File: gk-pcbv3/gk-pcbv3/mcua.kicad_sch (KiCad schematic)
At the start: 24 parts, among them J14 Conn_01x02, SW1 SW_Push, U4 STM32H747BITx, Y1 16MHz, Y2 32.768kHz R26-32.768-12.5

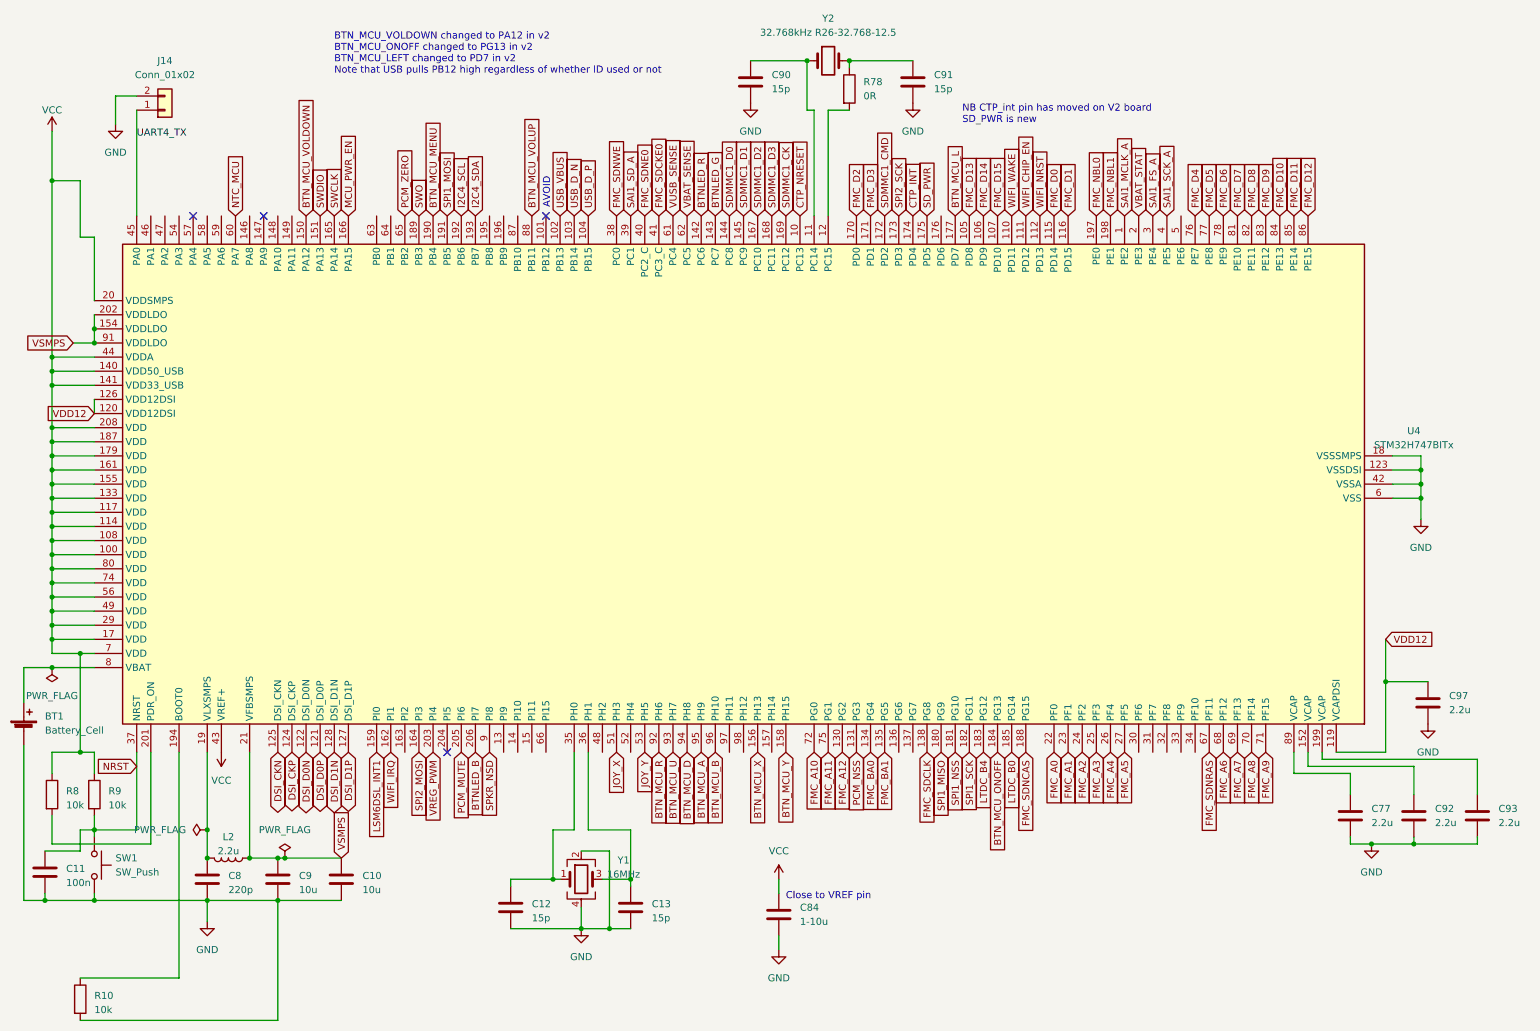
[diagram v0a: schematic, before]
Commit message: v3 board
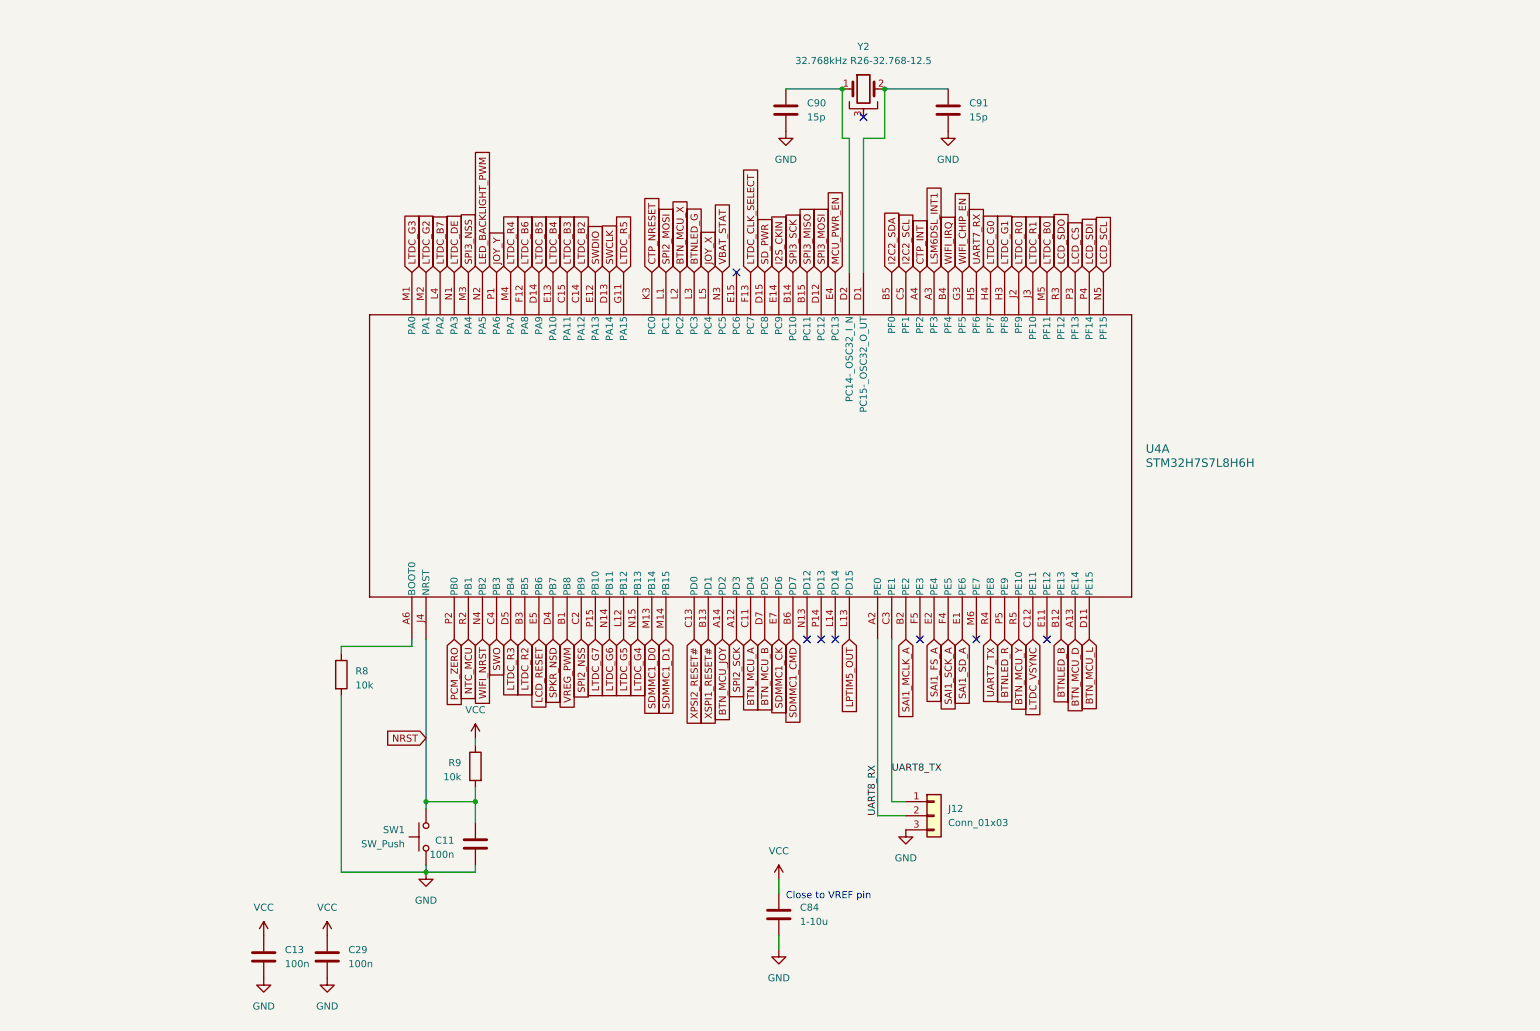
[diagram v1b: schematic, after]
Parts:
- removed BT1: Battery_Cell, Battery:BatteryHolder_Keystone_3002_1x2032, symbol Device:Battery_Cell
- removed C10, C9: 10u, Capacitor_SMD:C_0805_2012Metric, symbol Device:C
- removed C12: 15p, Capacitor_SMD:C_0603_1608Metric, symbol Device:C
- removed C77, C92, C93: 2.2u, Capacitor_SMD:C_0603_1608Metric, symbol Device:C
- removed C8: 220p, Capacitor_SMD:C_0603_1608Metric, symbol Device:C
- removed C97: 2.2u, Capacitor_SMD:C_0805_2012Metric, symbol Device:C
- removed J14: Conn_01x02, Connector_PinHeader_2.54mm:PinHeader_1x02_P2.54mm_Vertical, symbol Connector_Generic:Conn_01x02
- removed L2: 2.2u, Inductor_SMD:L_7.3x7.3_H3.5, symbol Device:L
- removed R10: 10k, Resistor_SMD:R_0603_1608Metric, symbol Device:R
- removed R78: 0R, Resistor_SMD:R_0603_1608Metric, symbol Device:R
- removed U4: STM32H747BITx, Package_QFP:LQFP-208_28x28mm_P0.5mm, symbol MCU_ST_STM32H7:STM32H747BITx
- removed Y1: 16MHz, Crystal:Crystal_SMD_SeikoEpson_TSX3225-4Pin_3.2x2.5mm, symbol Device:Crystal_GND24
- added C29: 100n, Capacitor_SMD:C_0603_1608Metric, symbol Device:C
- added J12: Conn_01x03, Connector_PinHeader_2.54mm:PinHeader_1x03_P2.54mm_Vertical, symbol Connector_Generic:Conn_01x03
- added U4: STM32H7S7L8H6H, STM32H7S7:TFBGA225_STM, symbol STM32 v2:STM32H7S7L8H6H
- C13: value 15p -> 100n
- Y2: symbol Device:Crystal -> Device:Crystal_GND3
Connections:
- net BTNLED_B: now also U4.B12 (PE13)
- net BTNLED_G: now also U4.L3 (PC3)
- net BTNLED_R: now also U4.P5 (PE9)
- net BTN_MCU_A: now also U4.C11 (PD4)
- net BTN_MCU_B: now also U4.D7 (PD5)
- net BTN_MCU_D: now also U4.A13 (PE14)
- net BTN_MCU_L: now also U4.D11 (PE15)
- net BTN_MCU_X: now also U4.L2 (PC2)
- net BTN_MCU_Y: now also U4.R5 (PE10)
- net CTP_INT: now also U4.A4 (PF2)
- net CTP_NRESET: now also U4.K3 (PC0)
- net GND: now also R8.2, C29.2, J12.3 (Pin_3)
- net JOY_X: now also U4.L5 (PC4)
- net JOY_Y: now also U4.P1 (PA6)
- net LSM6DSL_INT1: now also U4.A3 (PF3)
- net LTDC_B0: now also U4.M5 (PF11)
- net LTDC_B4: now also U4.E13 (PA10)
- net MCU_PWR_EN: now also U4.E4 (PC13)
- net NRST: now also U4.J4 (NRST)
- net NTC_MCU: now also U4.R2 (PB1)
- net PCM_ZERO: now also U4.P2 (PB0)
- net SAI1_FS_A: now also U4.E2 (PE4)
- net SAI1_MCLK_A: now also U4.B2 (PE2)
- net SAI1_SCK_A: now also U4.F4 (PE5)
- net SAI1_SD_A: now also U4.E1 (PE6)
- net SDMMC1_CK: now also U4.E7 (PD6)
- net SDMMC1_CMD: now also U4.B6 (PD7)
- net SDMMC1_D0: now also U4.M13 (PB14)
- net SDMMC1_D1: now also U4.M14 (PB15)
- net SD_PWR: now also U4.D15 (PC8)
- net SPI2_MOSI: now also U4.L1 (PC1)
- net SPI2_SCK: now also U4.A12 (PD3)
- net SPKR_NSD: now also U4.D4 (PB7)
- net SWCLK: now also U4.D13 (PA14)
- net SWDIO: now also U4.E12 (PA13)
- net SWO: now also U4.C4 (PB3)
- net VBAT_STAT: now also U4.N3 (PC5)
- net VCC: now also C13.1, C29.1; no longer R8.1
- net VREG_PWM: now also U4.B1 (PB8)
- net WIFI_CHIP_EN: now also U4.G3 (PF5)
- net WIFI_IRQ: now also U4.B4 (PF4)
- net WIFI_NRST: now also U4.N4 (PB2)
- net at C91.1, Y2.2: now also U4.D1 (PC15-_OSC32_O_UT)
- net at C90.1, Y2.1: now also U4.D2 (PC14-_OSC32_I_N)
- new net: R8.1, U4.A6 (BOOT0)
- new net BTN_MCU_JOY: U4.A14 (PD2)
- new net I2C2_SCL: U4.C5 (PF1)
- new net I2C2_SDA: U4.B5 (PF0)
- new net I2S_CKIN: U4.E14 (PC9)
- new net LCD_CS: U4.P3 (PF13)
- new net LCD_RESET: U4.E5 (PB6)
- new net LCD_SCL: U4.N5 (PF15)
- new net LCD_SDI: U4.P4 (PF14)
- new net LCD_SDO: U4.R3 (PF12)
- new net LED_BACKLIGHT_PWM: U4.N2 (PA5)
- new net LPTIM5_OUT: U4.L13 (PD15)
- new net LTDC_B2: U4.C14 (PA12)
- new net LTDC_B3: U4.C15 (PA11)
- new net LTDC_B5: U4.D14 (PA9)
- new net LTDC_B6: U4.F12 (PA8)
- new net LTDC_B7: U4.L4 (PA2)
- new net LTDC_CLK_SELECT: U4.F13 (PC7)
- new net LTDC_DE: U4.N1 (PA3)
- new net LTDC_G0: U4.H4 (PF7)
- new net LTDC_G1: U4.H3 (PF8)
- new net LTDC_G2: U4.M2 (PA1)
- new net LTDC_G3: U4.M1 (PA0)
- new net LTDC_G4: U4.N15 (PB13)
- new net LTDC_G5: U4.L12 (PB12)
- new net LTDC_G6: U4.N14 (PB11)
- new net LTDC_G7: U4.P15 (PB10)
- new net LTDC_R0: U4.J2 (PF9)
- new net LTDC_R1: U4.J3 (PF10)
- new net LTDC_R2: U4.B3 (PB5)
- new net LTDC_R3: U4.D5 (PB4)
- new net LTDC_R4: U4.M4 (PA7)
- new net LTDC_R5: U4.G11 (PA15)
- new net LTDC_VSYNC: U4.C12 (PE11)
- new net SPI2_NSS: U4.C2 (PB9)
- new net SPI3_MISO: U4.B15 (PC11)
- new net SPI3_MOSI: U4.D12 (PC12)
- new net SPI3_NSS: U4.M3 (PA4)
- new net SPI3_SCK: U4.B14 (PC10)
- new net UART7_RX: U4.H5 (PF6)
- new net UART7_TX: U4.R4 (PE8)
- new net UART8_RX: J12.2 (Pin_2), U4.A2 (PE0)
- new net UART8_TX: J12.1 (Pin_1), U4.C3 (PE1)
- new net XPSI2_RESET#: U4.C13 (PD0)
- new net XSPI1_RESET#: U4.B13 (PD1)
- no-connect marks 4 -> 8
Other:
- note removed: "AVOID"
- note removed: "BTN_MCU_VOLDOWN changed to PA12 in v2 BTN_MCU_ONOFF changed to PG13 in v2 BTN_MCU_LEFT changed to PD7 in v2 Note that USB pulls PB12 high regardless of whether ID used or not"
- note removed: "NB CTP_int pin has moved on V2 board SD_PWR is new"
- moved on the sheet: C11, C90, C91, R8, R9, SW1
